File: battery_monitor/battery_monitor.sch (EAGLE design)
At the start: 7 parts

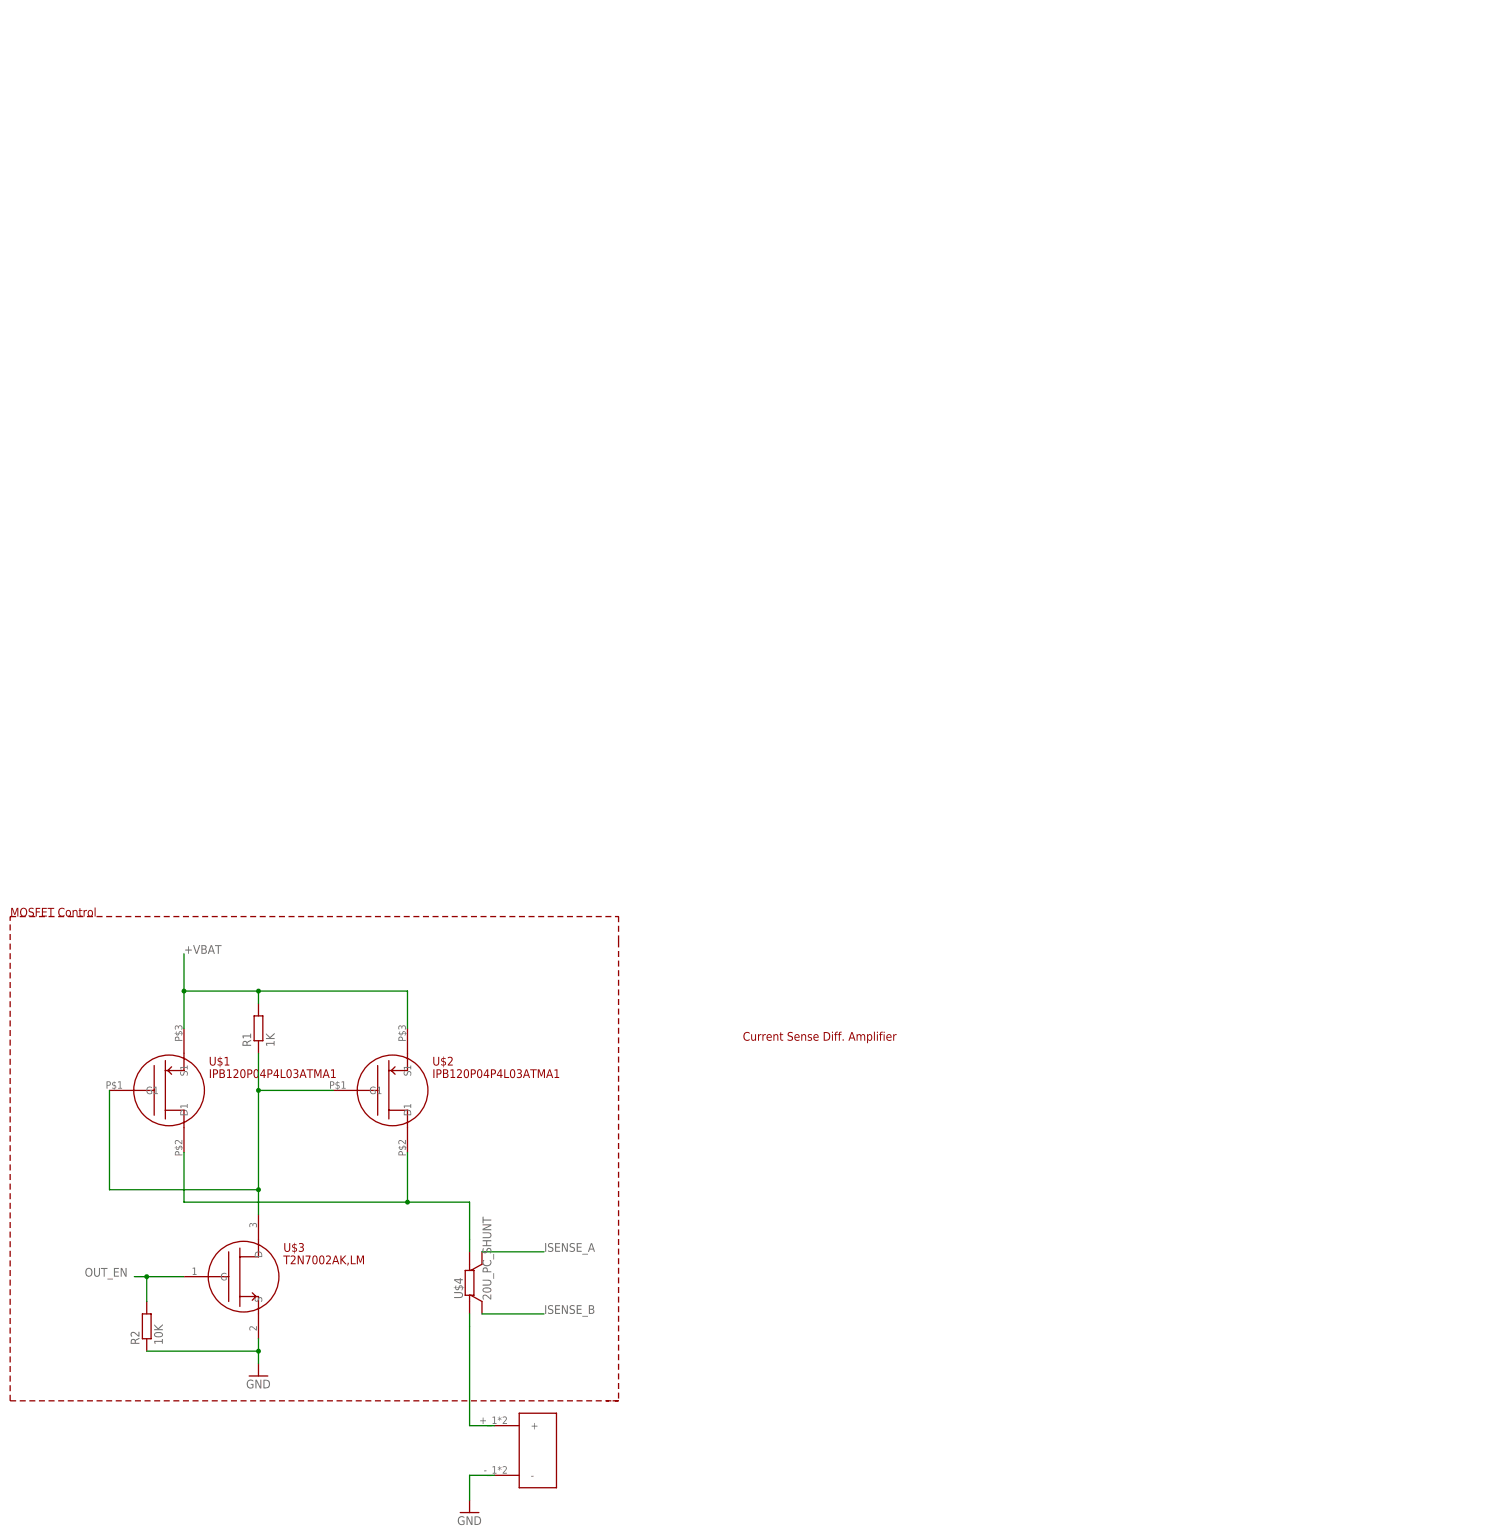
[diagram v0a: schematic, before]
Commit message: Finished design block
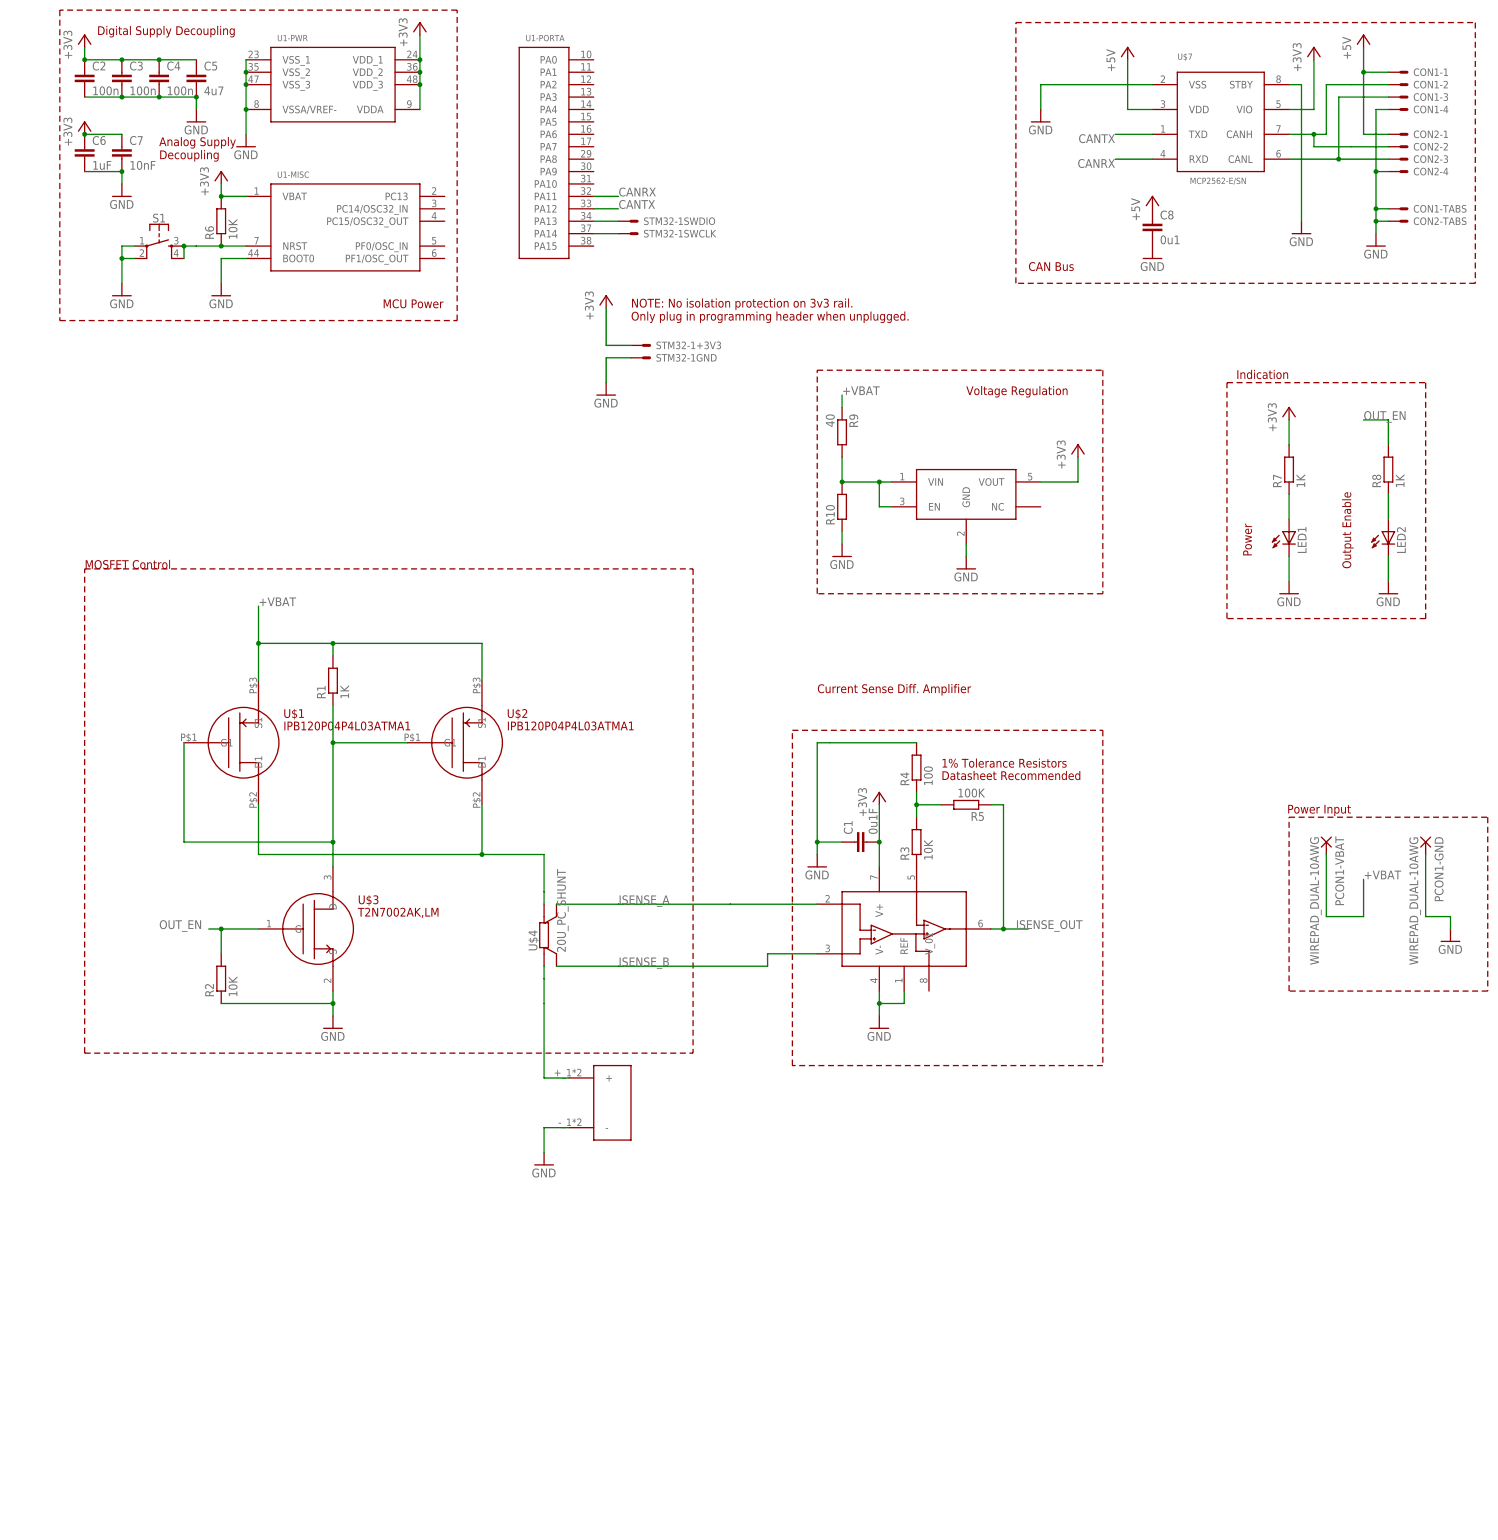
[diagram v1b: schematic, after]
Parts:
- added C1: 0u1F, resistor:C-EUC0805
- added C2, C3, C4: 100n, resistor:C-EUC0805
- added C5: 4u7, resistor:C-EUC0805
- added C6: 1uF, resistor:C-EUC0805
- added C7: 10nF, resistor:C-EUC0805
- added C8: 0u1, resistor:C-EUC0805
- added CON1, CON2: SM04B-GHS-TB, SPEAR-general:SM04B-GHS-TB
- added LED1, LED2: (no value), led:LEDCHIPLED_0805
- added PCON1: WIREPAD_DUAL-10AWG, SPEAR-battery-monitor:WIREPAD_DUAL-10AWG
- added R10: (no value), resistor:R-EU_R0805
- added R3, R6: 10K, resistor:R-EU_R0805
- added R4: 100, resistor:R-EU_R0805
- added R5: 100K, resistor:R-EU_R0805
- added R7, R8: 1K, resistor:R-EU_R0805
- added R9: 40, resistor:R-EU_R0805
- added S1: (no value), SPEAR-arm-control:MOMENTARY-SWITCH-SPST-2-SMD-4.6X2.8MM
- added STM32-1: STM32_SWD-HDR, SPEAR-battery-monitor:STM32_SWD-HDR
- added U$6: INA145, SPEAR-battery-monitor:INA145
- added U$7: MCP2562-E/SN, SPEAR-general:MCP2562-E/SN
- added U$8: LP2981, SPEAR-battery-monitor:LP2981
- added U1: STM32F303CB, SPEAR-general:STM32F303CB
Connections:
- new net +3V3: C1.2, C2.1, C3.1, C4.1, C5.1, C6.1, C7.1, R6.2, R7.2, STM32-1+3V3.S, U$6.V+, U$7.VIO, U$8.VOUT, U1-MISC.VBAT, U1-PWR.VDDA, U1-PWR.VDD_1, U1-PWR.VDD_2, U1-PWR.VDD_3
- new net +5V: C8.1, CON1-1.S, CON2-1.S, U$7.VDD
- new net CANH: CON1-2.S, CON2-2.S, U$7.CANH
- new net CANL: CON1-3.S, CON2-3.S, U$7.CANL
- new net CANRX: U$7.RXD, U1-PORTA.PA11
- new net CANTX: U$7.TXD, U1-PORTA.PA12
- new net ISENSE_OUT: R5.1, U$6.OUT
- new net N$3: R3.1, U$6.VG
- new net N$4: R3.2, R4.1, R5.2
- new net N$5: STM32-1SWDIO.S, U1-PORTA.PA13
- new net N$6: STM32-1SWCLK.S, U1-PORTA.PA14
- new net N$7: LED1.A, R7.1
- new net N$8: R10.2, R9.2, U$8.EN, U$8.VIN
- new net N$9: LED2.A, R8.1
- new net NRST: R6.1, S1.3, S1.4, U1-MISC.NRST
- net +VBAT: now also PCON1-VBAT.P, R9.1
- net GND: now also C1.1, C2.2, C3.2, C4.2, C5.2, C6.2, C7.2, C8.2, CON1-4.S, CON1-TABS.S, CON2-4.S, CON2-TABS.S, LED1.C, LED2.C, PCON1-GND.P, R10.1, R4.2, S1.1, S1.2, STM32-1GND.S, U$6.REF, U$6.V-, U$7.STBY, U$7.VSS, U$8.GND, U1-MISC.BOOT0, U1-PWR.VSSA/VREF-, U1-PWR.VSS_1, U1-PWR.VSS_2, U1-PWR.VSS_3
- net ISENSE_A: now also U$6.IN-
- net ISENSE_B: now also U$6.IN+
- net OUT_EN: now also R8.2
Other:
- note added: "1% Tolerance Resistors"
- note added: "Analog Supply Decoupling"
- note added: "CAN Bus"
- note added: "Datasheet Recommended"
- note added: "Digital Supply Decoupling"
- note added: "Indication"
- note added: "MCU Power"
- note added: "NOTE: No isolation protection on 3v3 rail. Only plug in programming header when unplugged."
- note added: "Output Enable"
- note added: "Power"
- note added: "Power Input"
- note added: "Voltage Regulation"
- moved on the sheet: R1, R2, U$1, U$2, U$3, U$4
